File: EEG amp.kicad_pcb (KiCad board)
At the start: 2 copper layers, 53 x 42.2 mm, 40 parts, among them J1 Electrodes, J2 Power, J3 Output, J4 Status, U1 AD8232, U2 TMUX154EDGS

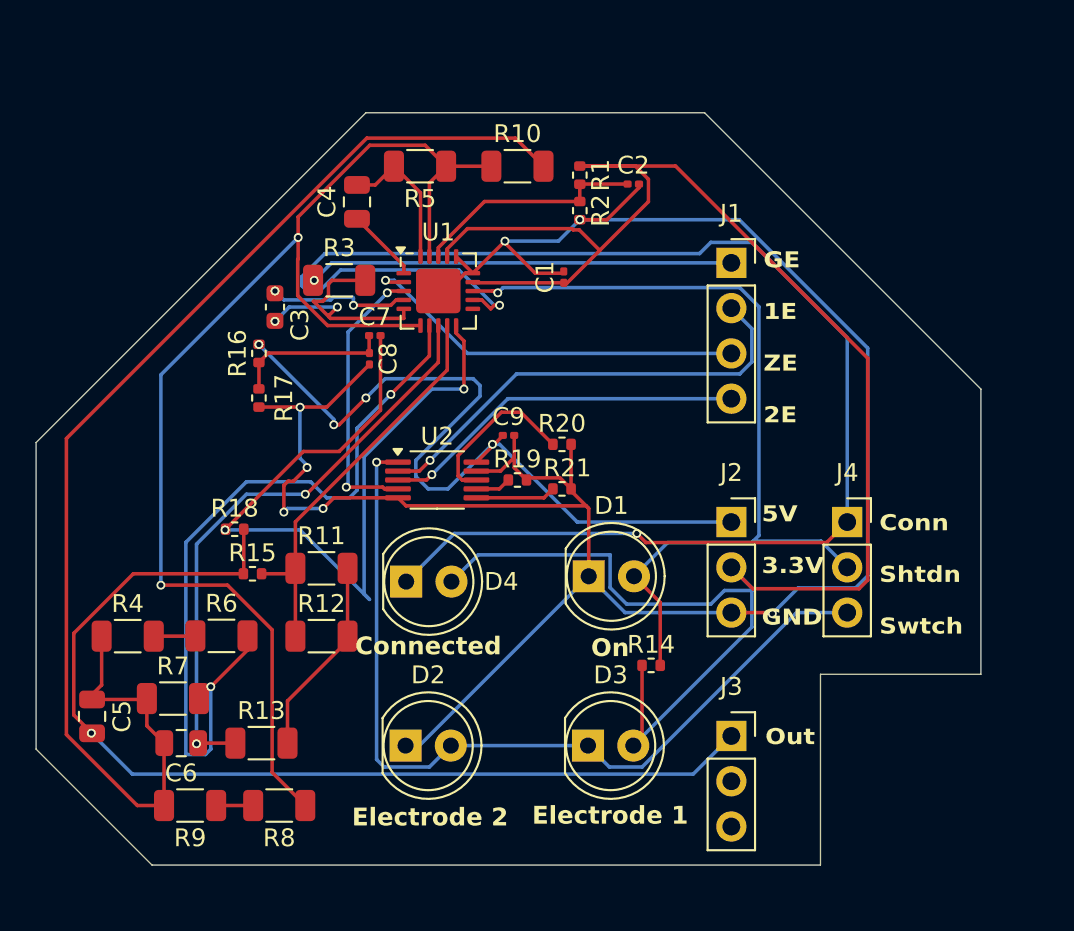
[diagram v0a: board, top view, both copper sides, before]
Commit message: Messed with schematic and(I think) finished PCB
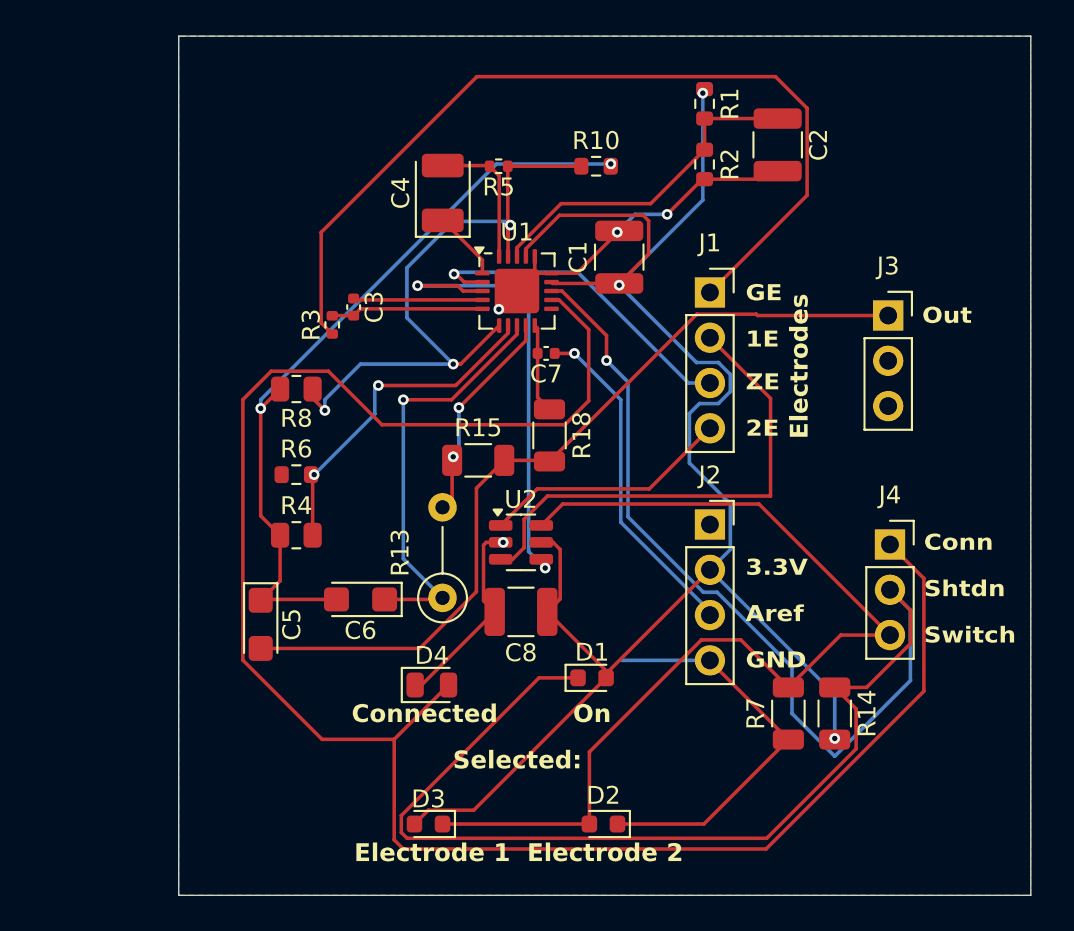
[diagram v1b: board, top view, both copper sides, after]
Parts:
- removed C9: 100nF, Capacitor_SMD:C_0201_0603Metric
- removed R11, R12: 33k, Resistor_SMD:R_1206_3216Metric
- removed R16, R17: 10k ±0.1%, Resistor_SMD:R_0402_1005Metric
- removed R19, R20, R21: 50R, Resistor_SMD:R_0402_1005Metric
- removed R9: 150, Resistor_SMD:R_1206_3216Metric
- C1, C2, C8: value 0.1uF -> ECHU1C104GX5; footprint Capacitor_SMD:C_0201_0603Metric -> Capacitor_SMD:C_1210_3225Metric
- C3: value 1nF -> CC0402JRX7R9BB102; footprint Capacitor_SMD:C_0603_1608Metric -> Capacitor_SMD:C_0402_1005Metric
- C4: value 100uF -> CA45-B6R3K107T; footprint Capacitor_SMD:C_0805_2012Metric -> Capacitor_Tantalum_SMD:CP_EIA-3528-21_Kemet-B
- C5, C6: value 10uF -> CA45-A010K106T; footprint Capacitor_SMD:C_0805_2012Metric -> Capacitor_Tantalum_SMD:CP_EIA-3216-12_Kemet-S
- C7: value 14pF -> 0402CG140J500NT; footprint Capacitor_SMD:C_0201_0603Metric -> Capacitor_SMD:C_0402_1005Metric
- D1: value Green -> XL-1608UBC-04; footprint LED_THT:LED_D5.0mm -> LED_SMD:LED_0603_1608Metric
- D2: value Yellow - 2e -> XL-1608UGC-04; footprint LED_THT:LED_D5.0mm -> LED_SMD:LED_0603_1608Metric
- D3: value Yellow - 1e -> XL-1608UGC-04; footprint LED_THT:LED_D5.0mm -> LED_SMD:LED_0603_1608Metric
- D4: value Red -> XL-2012UWC; footprint LED_THT:LED_D5.0mm -> LED_SMD:LED_0805_2012Metric
- J2: footprint Connector_PinSocket_2.54mm:PinSocket_1x03_P2.54mm_Vertical -> Connector_PinSocket_2.54mm:PinSocket_1x04_P2.54mm_Vertical
- R1, R2: value 10k ±0.1% -> ARG03BTC1002; footprint Resistor_SMD:R_0402_1005Metric -> Resistor_SMD:R_0603_1608Metric
- R10: value 33k -> 0603WAD3302T5E; footprint Resistor_SMD:R_1206_3216Metric -> Resistor_SMD:R_0603_1608Metric
- R13: value 1k -> CF1/6W-7.5KΩ±5%T52; footprint Resistor_SMD:R_1206_3216Metric -> Resistor_THT:R_Axial_DIN0207_L6.3mm_D2.5mm_P5.08mm_Vertical
- R14, R15, R18: value 10k -> 1206W4F1002T5E; footprint Resistor_SMD:R_0402_1005Metric -> Resistor_SMD:R_1206_3216Metric
- R3, R5: value 330k -> SCR0402J330K; footprint Resistor_SMD:R_1206_3216Metric -> Resistor_SMD:R_0402_1005Metric
- R4, R8: value 10 -> ARG05DTC1600; footprint Resistor_SMD:R_1206_3216Metric -> Resistor_SMD:R_0805_2012Metric
- R6: value 150 -> 0603WAD3302T5E; footprint Resistor_SMD:R_1206_3216Metric -> Resistor_SMD:R_0603_1608Metric
- R7: value 33k -> 1206W4F1002T5E
- U2: value TMUX154EDGS -> TS5A3159ADBVR; footprint Package_SO:VSSOP-10_3x3mm_P0.5mm -> Package_TO_SOT_SMD:SOT-23-6
- moved R7 34.5 mm to (170.2, 112.2), turned to 90 degrees
- moved J3 25.2 mm to (175.8, 89.9)
- moved R8 23.4 mm to (142.6, 94.0)
- moved R18 18.4 mm to (156.8, 96.6), turned to -90 degrees
- moved C8 16.5 mm to (155.2, 106.5), turned to 180 degrees
- moved R15 14.2 mm to (152.8, 98.0)
- moved R13 13.0 mm to (150.8, 105.7), turned to 90 degrees
- moved C6 12.9 mm to (146.2, 105.8)
- moved D2 11.9 mm to (159.8, 118.4), turned to 180 degrees
- moved R4 11.0 mm to (142.6, 102.2)
- moved C5 10.8 mm to (140.6, 107.2)
- moved R14 10.6 mm to (172.8, 112.2), turned to -90 degrees
- moved R6 9.97 mm to (142.6, 98.8)
- moved D3 9.97 mm to (150.0, 118.4), turned to 180 degrees
- moved C7 9.66 mm to (156.6, 92.0), turned to 180 degrees
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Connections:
- C8 pad 1: Aref -> +3.3V
- D1 pad 1: GND -> shutdown
- D1 pad 2: shutdown -> +3.3V
- D4 pad 1: connected1 -> GND
- D4 pad 2: +3.3V -> connected1
- J2 pad 1: +5V -> unconnected-(J2-Pin_1-Pad1)
- J2 pad 3: GND -> Aref
- R13 pad 2: Net-(R11-Pad2) -> OPAMP-1
- R14 pad 1: +3.3V -> shutdown
- R14 pad 2: shutdown -> +3.3V
- R15 pad 1: 1o -> OPAMP-1
- R15 pad 2: OPAMP-1 -> 1o
- R4 pad 2: Net-(R4-Pad2) -> OPAMP+1
- R6 pad 1: Net-(R4-Pad2) -> Net-(C5-Pad1)
- R7 pad 1: Net-(C5-Pad1) -> GND
- R7 pad 2: OPAMP+1 -> switch
- R8 pad 2: Net-(R8-Pad2) -> Net-(C5-Pad1)
- U2 pad 1: switch -> 2e
- U2 pad 2: 1e -> GND
- U2 pad 3: 2e -> 1e
- U2 pad 5: GND -> +3.3V
- U2 pad 6: Net-(U2-B) -> switch
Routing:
- net GND: track 130.2 -> 50.0 mm, vias 7 -> 4
- net shutdown: track 49.1 -> 99.5 mm
- net +5V: track 45.3 -> 0.00 mm, vias 4 -> 0
- net UFOUT1: track 44.4 -> 5.04 mm, vias 2 -> 0
- net IAOUT1: track 71.0 -> 36.9 mm, vias 2 -> 3
- net Net-(C5-Pad1): track 71.4 -> 43.0 mm, vias 0 -> 2
- net Ge: track 23.8 -> 50.2 mm, vias 1 -> 0
- net OPAMP+1: track 44.0 -> 18.7 mm
- net connected1: track 85.4 -> 106.1 mm, vias 2 -> 0
- net Ie: track 15.8 -> 27.1 mm
- net Net-(R11-Pad2): track 11.2 -> 0.00 mm
- net OPAMP-1: track 23.0 -> 11.9 mm, vias 0 -> 2
- net 1o: track 57.2 -> 46.4 mm, vias 1 -> 0
- net +3.3V: track 106.2 -> 96.2 mm, vias 0 -> 3
- net Aref: track 8.89 -> 18.7 mm, vias 0 -> 1
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- added copper zone on B.Cu, net GND
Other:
- board size 53 x 42.2 mm -> 47.8 x 48.2 mm
- board text added: "1E"
- board text added: "2E"
- board text added: "3.3V"
- board text added: "Aref"
- board text added: "Conn"
- board text added: "Electrodes"
- board text added: "GE"
- board text added: "GND"
- board text added: "Selected:"
- board text added: "Shtdn"
- board text added: "Switch"
- board text added: "ZE"
- board text removed: "5V 3.3V GND"
- board text removed: "Conn Shtdn Swtch"
- board text removed: "GE 1E ZE 2E"
